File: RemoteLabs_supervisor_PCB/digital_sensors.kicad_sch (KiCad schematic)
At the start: 8 parts, among them J23 limit_switch_A, J24 limit_switch_B, J25 Optical Encoder

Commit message: Schematic reviewed
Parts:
- J23, J24: footprint (none) -> Connector_PinHeader_2.54mm:PinHeader_1x02_P2.54mm_Vertical
- J25: footprint Connector_PinHeader_1.27mm:PinHeader_1x05_P1.27mm_Vertical -> Connector_PinHeader_2.54mm:PinHeader_1x05_P2.54mm_Vertical
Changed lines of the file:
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@@
     (property "Reference" "J23" (id 0) (at 88.265 40.64 0))
     (property "Value" "limit_switch_A" (id 1) (at 88.265 43.18 0))
-    (property "Footprint" "" (id 2) (at 87.63 45.72 0)
+    (property "Footprint" "Connector_PinHeader_2.54mm:PinHeader_1x02_P2.54mm_Vertical" (id 2) (at 87.63 45.72 0)
       (effects (font (size 1.27 1.27)) hide)
     )
@@
     (property "Reference" "J25" (id 0) (at 78.74 95.25 0))
     (property "Value" "Optical Encoder" (id 1) (at 85.09 97.79 0))
-    (property "Footprint" "Connector_PinHeader_1.27mm:PinHeader_1x05_P1.27mm_Vertical" (id 2) (at 87.63 106.68 0)
+    (property "Footprint" "Connector_PinHeader_2.54mm:PinHeader_1x05_P2.54mm_Vertical" (id 2) (at 87.63 106.68 0)
       (effects (font (size 1.27 1.27)) hide)
     )
@@
     (pin "2")
   )
-  (symbol (lib_id "Connector:Conn_01x02_Male") (at 87.63 55.88 0) (unit 1)
+  (symbol (lib_name "Conn_01x02_Male_1") (lib_id "Connector:Conn_01x02_Male") (at 87.63 55.88 0) (unit 1)
     (in_bom yes) (on_board yes) (fields_autoplaced)
     (property "Reference" "J24" (id 0) (at 88.265 50.8 0))
     (property "Value" "limit_switch_B" (id 1) (at 88.265 53.34 0))
-    (property "Footprint" "" (id 2) (at 87.63 55.88 0)
+    (property "Footprint" "Connector_PinHeader_2.54mm:PinHeader_1x02_P2.54mm_Vertical" (id 2) (at 87.63 55.88 0)
       (effects (font (size 1.27 1.27)) hide)
     )

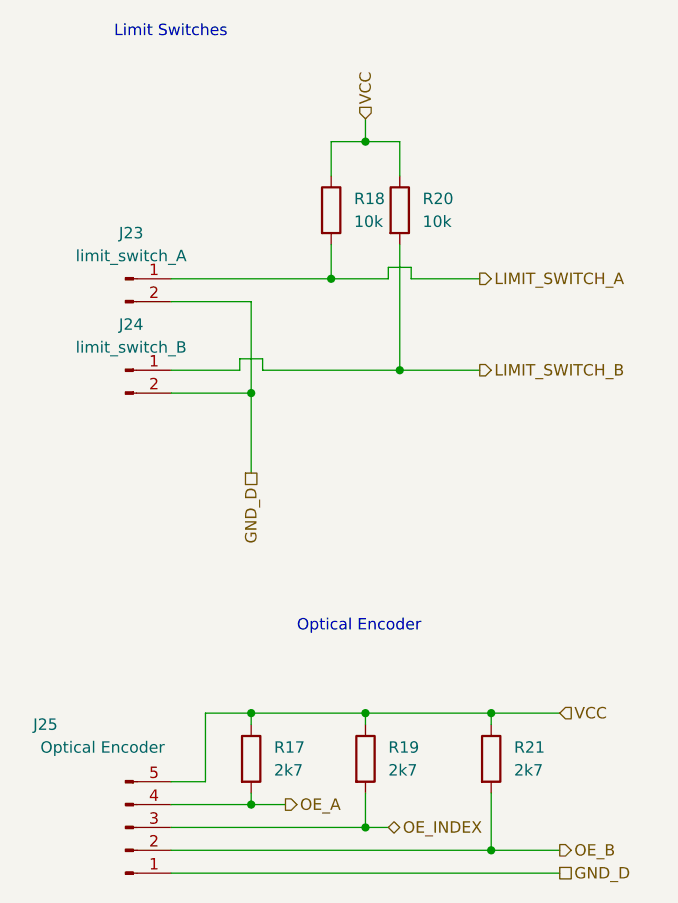
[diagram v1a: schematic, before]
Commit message: mbncmvbc,
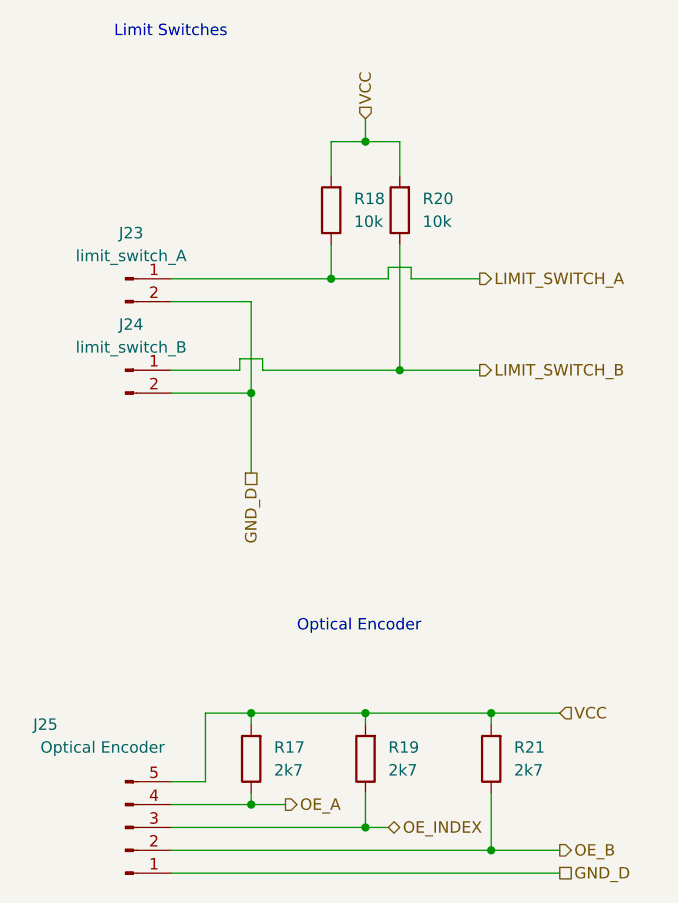
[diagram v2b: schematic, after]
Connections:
- net LIMIT_SWITCH_A: now also R18.1; no longer R18.2
- net LIMIT_SWITCH_B: now also R20.1; no longer R20.2
- net OE_A: now also R17.1; no longer R17.2
- net OE_B: now also R21.1; no longer R21.2
- net OE_INDEX: now also R19.1; no longer R19.2
- net VCC: now also R17.2, R18.2, R19.2, R20.2, R21.2; no longer R17.1, R18.1, R19.1, R20.1, R21.1
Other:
- moved on the sheet: R17, R18, R19, R20, R21
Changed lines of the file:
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@@
     (effects (font (size 1.27 1.27)) (justify left))
   )
-  (symbol (lib_id "000_Resistors_Immo:Resistor_0805") (at 128.27 99.06 0) (unit 1)
+  (symbol (lib_id "000_Resistors_Immo:Resistor_0805") (at 128.27 99.06 90) (unit 1)
     (in_bom yes) (on_board yes) (fields_autoplaced)
-    (property "Reference" "R21" (id 0) (at 130.81 97.7899 0)
-      (effects (font (size 1.27 1.27)) (justify left))
+    (property "Reference" "R21" (id 0) (at 130.81 97.7899 90)
+      (effects (font (size 1.27 1.27)) (justify right))
     )
-    (property "Value" "2k7" (id 1) (at 130.81 100.3299 0)
-      (effects (font (size 1.27 1.27)) (justify left))
+    (property "Value" "2k7" (id 1) (at 130.81 100.3299 90)
+      (effects (font (size 1.27 1.27)) (justify right))
     )
-    (property "Footprint" "Resistor_SMD:R_0805_2012Metric_Pad1.20x1.40mm_HandSolder" (id 2) (at 126.492 99.06 90)
+    (property "Footprint" "Resistor_SMD:R_0805_2012Metric_Pad1.20x1.40mm_HandSolder" (id 2) (at 128.27 100.838 90)
       (effects (font (size 1.27 1.27)) hide)
     )
@@
     (pin "2")
   )
-  (symbol (lib_id "000_Resistors_Immo:Resistor_0805") (at 101.6 99.06 0) (unit 1)
+  (symbol (lib_id "000_Resistors_Immo:Resistor_0805") (at 101.6 99.06 90) (unit 1)
     (in_bom yes) (on_board yes) (fields_autoplaced)
-    (property "Reference" "R17" (id 0) (at 104.14 97.7899 0)
-      (effects (font (size 1.27 1.27)) (justify left))
+    (property "Reference" "R17" (id 0) (at 104.14 97.7899 90)
+      (effects (font (size 1.27 1.27)) (justify right))
     )
-    (property "Value" "2k7" (id 1) (at 104.14 100.3299 0)
-      (effects (font (size 1.27 1.27)) (justify left))
+    (property "Value" "2k7" (id 1) (at 104.14 100.3299 90)
+      (effects (font (size 1.27 1.27)) (justify right))
     )
-    (property "Footprint" "Resistor_SMD:R_0805_2012Metric_Pad1.20x1.40mm_HandSolder" (id 2) (at 99.822 99.06 90)
+    (property "Footprint" "Resistor_SMD:R_0805_2012Metric_Pad1.20x1.40mm_HandSolder" (id 2) (at 101.6 100.838 90)
       (effects (font (size 1.27 1.27)) hide)
     )
@@
     (pin "2")
   )
-  (symbol (lib_id "000_Resistors_Immo:Resistor_0805") (at 118.11 38.1 0) (unit 1)
+  (symbol (lib_id "000_Resistors_Immo:Resistor_0805") (at 118.11 38.1 90) (unit 1)
     (in_bom yes) (on_board yes) (fields_autoplaced)
-    (property "Reference" "R20" (id 0) (at 120.65 36.8299 0)
-      (effects (font (size 1.27 1.27)) (justify left))
+    (property "Reference" "R20" (id 0) (at 120.65 36.8299 90)
+      (effects (font (size 1.27 1.27)) (justify right))
     )
-    (property "Value" "10k" (id 1) (at 120.65 39.3699 0)
-      (effects (font (size 1.27 1.27)) (justify left))
+    (property "Value" "10k" (id 1) (at 120.65 39.3699 90)
+      (effects (font (size 1.27 1.27)) (justify right))
     )
-    (property "Footprint" "Resistor_SMD:R_0805_2012Metric_Pad1.20x1.40mm_HandSolder" (id 2) (at 116.332 38.1 90)
+    (property "Footprint" "Resistor_SMD:R_0805_2012Metric_Pad1.20x1.40mm_HandSolder" (id 2) (at 118.11 39.878 90)
       (effects (font (size 1.27 1.27)) hide)
     )
@@
     (pin "2")
   )
-  (symbol (lib_id "000_Resistors_Immo:Resistor_0805") (at 114.3 99.06 0) (unit 1)
+  (symbol (lib_id "000_Resistors_Immo:Resistor_0805") (at 114.3 99.06 90) (unit 1)
     (in_bom yes) (on_board yes) (fields_autoplaced)
-    (property "Reference" "R19" (id 0) (at 116.84 97.7899 0)
-      (effects (font (size 1.27 1.27)) (justify left))
+    (property "Reference" "R19" (id 0) (at 116.84 97.7899 90)
+      (effects (font (size 1.27 1.27)) (justify right))
     )
-    (property "Value" "2k7" (id 1) (at 116.84 100.3299 0)
-      (effects (font (size 1.27 1.27)) (justify left))
+    (property "Value" "2k7" (id 1) (at 116.84 100.3299 90)
+      (effects (font (size 1.27 1.27)) (justify right))
     )
-    (property "Footprint" "Resistor_SMD:R_0805_2012Metric_Pad1.20x1.40mm_HandSolder" (id 2) (at 112.522 99.06 90)
+    (property "Footprint" "Resistor_SMD:R_0805_2012Metric_Pad1.20x1.40mm_HandSolder" (id 2) (at 114.3 100.838 90)
       (effects (font (size 1.27 1.27)) hide)
     )
@@
     (pin "5")
   )
-  (symbol (lib_id "000_Resistors_Immo:Resistor_0805") (at 110.49 38.1 0) (unit 1)
+  (symbol (lib_id "000_Resistors_Immo:Resistor_0805") (at 110.49 38.1 90) (unit 1)
     (in_bom yes) (on_board yes) (fields_autoplaced)
-    (property "Reference" "R18" (id 0) (at 113.03 36.8299 0)
-      (effects (font (size 1.27 1.27)) (justify left))
+    (property "Reference" "R18" (id 0) (at 113.03 36.8299 90)
+      (effects (font (size 1.27 1.27)) (justify right))
     )
-    (property "Value" "10k" (id 1) (at 113.03 39.3699 0)
-      (effects (font (size 1.27 1.27)) (justify left))
+    (property "Value" "10k" (id 1) (at 113.03 39.3699 90)
+      (effects (font (size 1.27 1.27)) (justify right))
     )
-    (property "Footprint" "Resistor_SMD:R_0805_2012Metric_Pad1.20x1.40mm_HandSolder" (id 2) (at 108.712 38.1 90)
+    (property "Footprint" "Resistor_SMD:R_0805_2012Metric_Pad1.20x1.40mm_HandSolder" (id 2) (at 110.49 39.878 90)
       (effects (font (size 1.27 1.27)) hide)
     )
@@
     (pin "2")
   )
-  (symbol (lib_name "Conn_01x02_Male_1") (lib_id "Connector:Conn_01x02_Male") (at 87.63 55.88 0) (unit 1)
+  (symbol (lib_id "Connector:Conn_01x02_Male") (at 87.63 55.88 0) (unit 1)
     (in_bom yes) (on_board yes) (fields_autoplaced)
     (property "Reference" "J24" (id 0) (at 88.265 50.8 0))

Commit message: PCB layout
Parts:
- J23, J24: footprint Connector_PinHeader_2.54mm:PinHeader_1x02_P2.54mm_Vertical -> Connector_Molex:Molex_KK-254_AE-6410-02A_1x02_P2.54mm_Vertical; symbol Connector:Conn_01x02_Male -> 000_Connectors_Immo:2pin_molex_2.54mm_male
- J25: footprint Connector_PinHeader_2.54mm:PinHeader_1x05_P2.54mm_Vertical -> Connector_Molex:Molex_KK-254_AE-6410-05A_1x05_P2.54mm_Vertical; symbol 000_Pin_Headers_Immo:Conn_01x05_Male -> 000_Pin_Headers_Immo:Molex_5pin_2.54mm_M
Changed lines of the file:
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@@
     (pin "2")
   )
-  (symbol (lib_id "Connector:Conn_01x02_Male") (at 87.63 45.72 0) (unit 1)
+  (symbol (lib_id "000_Connectors_Immo:2pin_molex_2.54mm_male") (at 87.63 45.72 0) (unit 1)
     (in_bom yes) (on_board yes) (fields_autoplaced)
     (property "Reference" "J23" (id 0) (at 88.265 40.64 0))
     (property "Value" "limit_switch_A" (id 1) (at 88.265 43.18 0))
-    (property "Footprint" "Connector_PinHeader_2.54mm:PinHeader_1x02_P2.54mm_Vertical" (id 2) (at 87.63 45.72 0)
+    (property "Footprint" "Connector_Molex:Molex_KK-254_AE-6410-02A_1x02_P2.54mm_Vertical" (id 2) (at 87.63 45.72 0)
       (effects (font (size 1.27 1.27)) hide)
     )
@@
     (pin "2")
   )
-  (symbol (lib_id "000_Pin_Headers_Immo:Conn_01x05_Male") (at 87.63 106.68 0) (mirror x) (unit 1)
+  (symbol (lib_id "000_Pin_Headers_Immo:Molex_5pin_2.54mm_M") (at 87.63 106.68 0) (mirror x) (unit 1)
     (in_bom yes) (on_board yes)
     (property "Reference" "J25" (id 0) (at 78.74 95.25 0))
     (property "Value" "Optical Encoder" (id 1) (at 85.09 97.79 0))
-    (property "Footprint" "Connector_PinHeader_2.54mm:PinHeader_1x05_P2.54mm_Vertical" (id 2) (at 87.63 106.68 0)
+    (property "Footprint" "Connector_Molex:Molex_KK-254_AE-6410-05A_1x05_P2.54mm_Vertical" (id 2) (at 89.535 96.52 0)
       (effects (font (size 1.27 1.27)) hide)
     )
@@
     (pin "2")
   )
-  (symbol (lib_id "Connector:Conn_01x02_Male") (at 87.63 55.88 0) (unit 1)
+  (symbol (lib_id "000_Connectors_Immo:2pin_molex_2.54mm_male") (at 87.63 55.88 0) (unit 1)
     (in_bom yes) (on_board yes) (fields_autoplaced)
     (property "Reference" "J24" (id 0) (at 88.265 50.8 0))
     (property "Value" "limit_switch_B" (id 1) (at 88.265 53.34 0))
-    (property "Footprint" "Connector_PinHeader_2.54mm:PinHeader_1x02_P2.54mm_Vertical" (id 2) (at 87.63 55.88 0)
+    (property "Footprint" "Connector_Molex:Molex_KK-254_AE-6410-02A_1x02_P2.54mm_Vertical" (id 2) (at 87.63 55.88 0)
       (effects (font (size 1.27 1.27)) hide)
     )
